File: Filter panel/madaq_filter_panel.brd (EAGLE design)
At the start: 70.6 x 38.2 mm, 34 parts

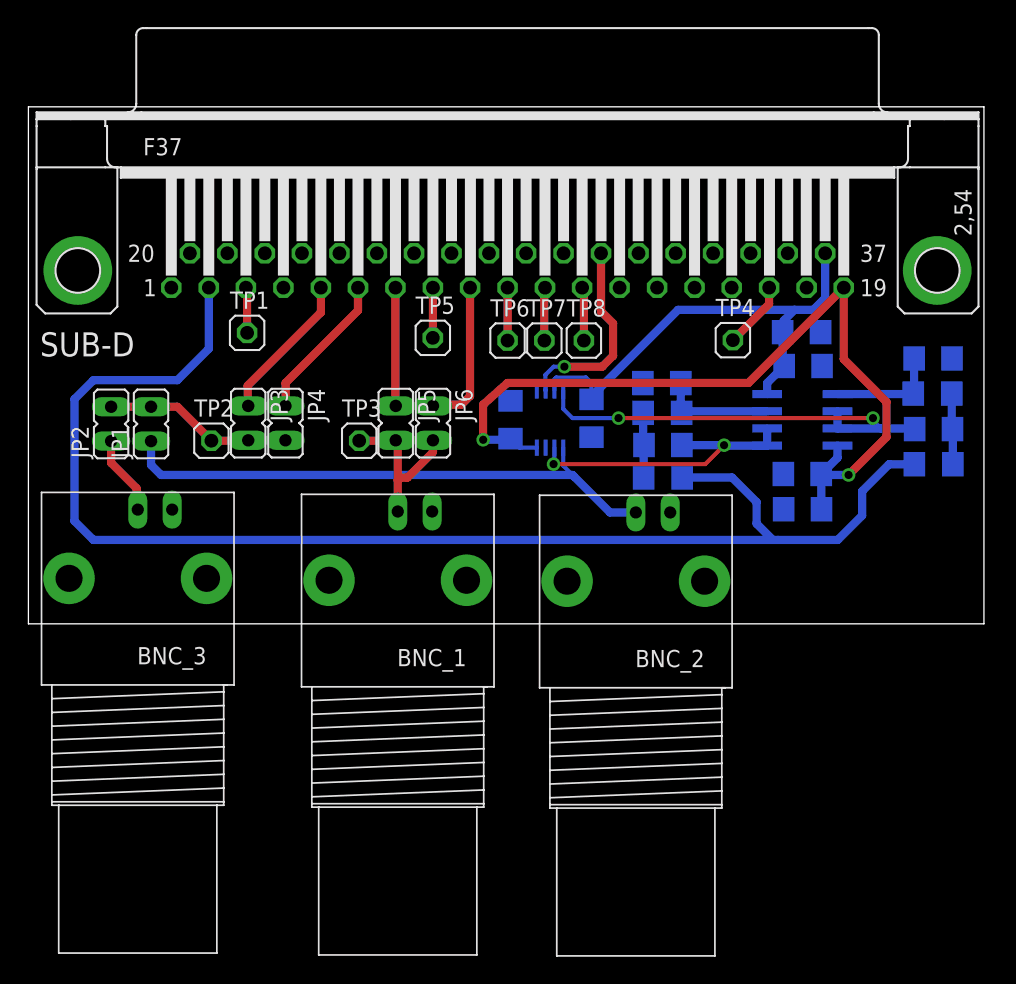
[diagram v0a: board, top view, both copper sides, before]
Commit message: Filter panel - V4 board (final?)
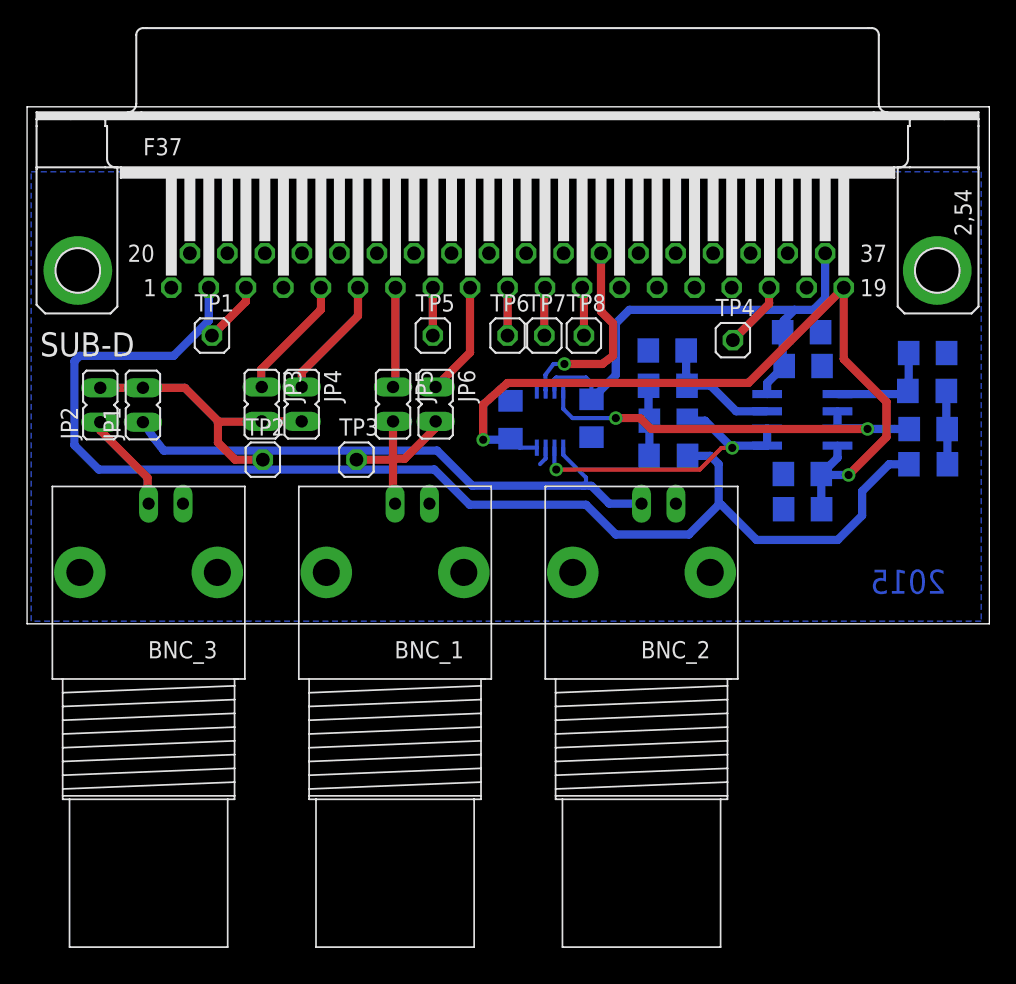
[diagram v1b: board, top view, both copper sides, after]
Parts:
- moved TP2 4.05 mm to (32.7, 53.3)
- moved TP1 2.61 mm to (29.0, 62.5)
- moved C6 2.43 mm to (62.6, 61.4)
- moved R1 2.04 mm to (62.6, 58.8)
- moved C5 1.84 mm to (62.7, 56.2)
- moved JP4 1.84 mm to (35.6, 57.4)
- moved JP3 1.72 mm to (32.6, 57.4)
- moved R2 1.65 mm to (62.7, 53.6)
- moved JP2 1.61 mm to (20.7, 57.4)
- moved JP1 1.52 mm to (23.9, 57.4)
- moved JP6 1.41 mm to (45.5, 57.4)
- moved TP3 1.41 mm to (39.6, 53.3)
- moved JP5 1.41 mm to (42.3, 57.4)
- moved BNC_3 0.91 mm to (24.3, 45.0)
- moved BNC_2 0.77 mm to (60.7, 45.0)
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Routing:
- net N$7: track 13.9 -> 21.3 mm
- net DAC_1: track 100.5 -> 95.1 mm
- net IN-4_B: track 11.1 -> 8.39 mm
- net -5V: track 35.9 -> 38.1 mm
- net IN-1_A: track 11.0 -> 9.06 mm
- net IN-0_A: track 11.0 -> 9.18 mm
- net SW_COM: track 41.5 -> 43.1 mm
- net SIG_1: track 22.0 -> 23.5 mm
- net GND: track 0.00 -> 1.39 mm
- net N$9: track 6.12 -> 7.50 mm
- net IN-2_A: track 8.75 -> 7.50 mm
- net DAC_2: track 3.38 -> 4.58 mm
- net SIG_2: track 32.5 -> 31.4 mm
- net N$8: track 12.4 -> 13.5 mm
- net N$3: track 8.24 -> 9.09 mm
- added copper zone on layer 16, net GND
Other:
- board size 70.6 x 38.2 mm -> 71.1 x 38.2 mm
- board text added: "2015"
- board text added: "DAC2"
- board text added: "DBG"
- board text added: "EXT"
- board text added: "IN0"
- board text added: "IN1"
- board text added: "IN2"
- board text added: "IN4"
- board text added: "INT"
